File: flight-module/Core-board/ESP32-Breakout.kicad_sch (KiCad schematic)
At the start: 18 parts, among them J10 USB4105-GF-A, J3 Probe_points, SW1 1825910-6, SW2 1825910-6, U10 ESP32-S3-WROOM-1-N16R2, U9 AZ1084-3.3

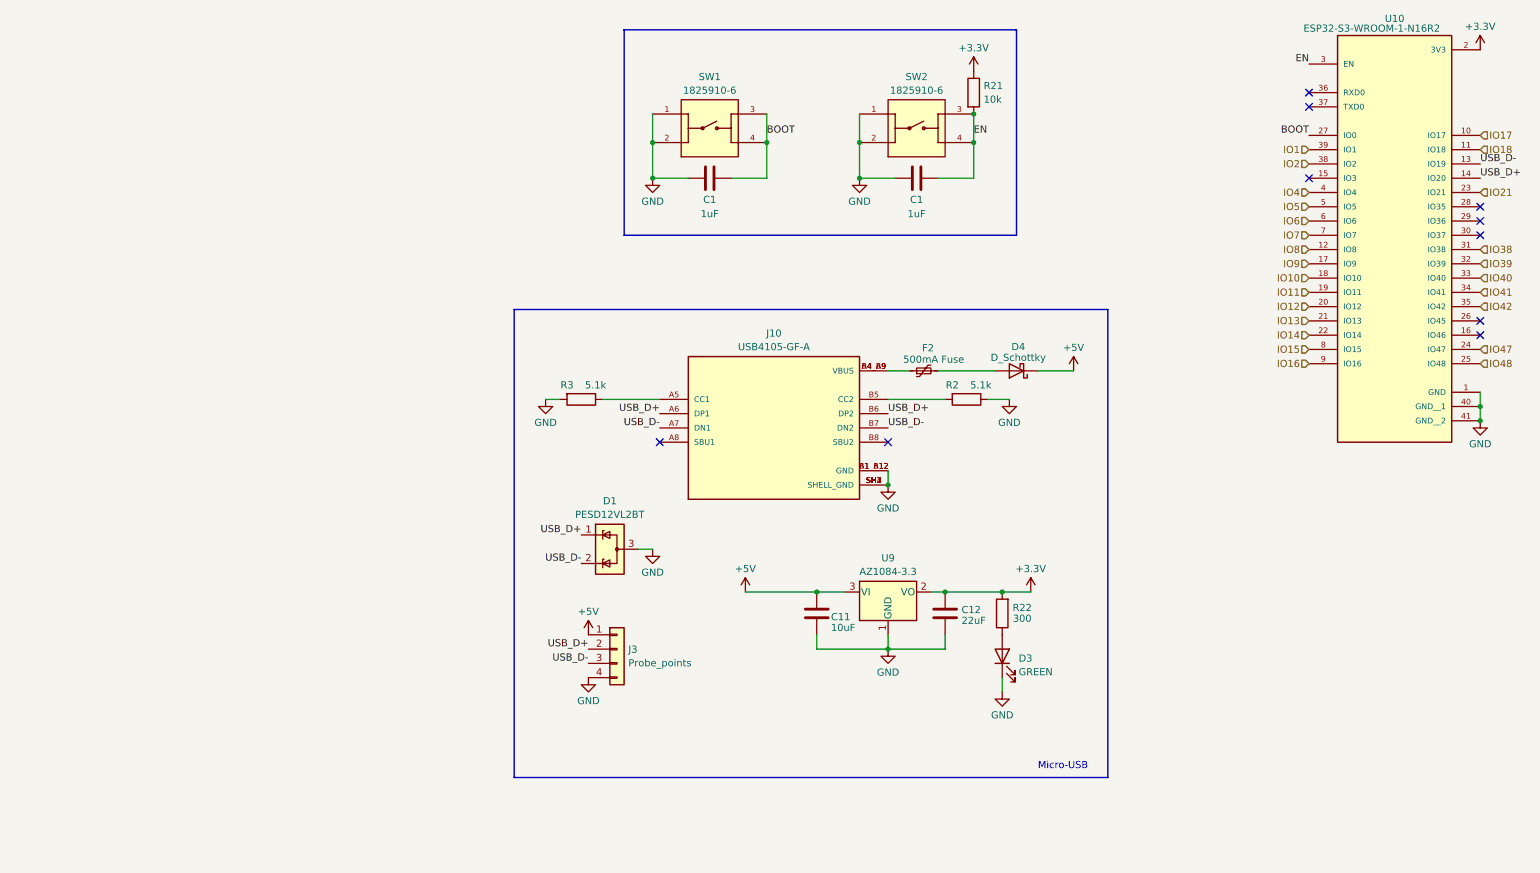
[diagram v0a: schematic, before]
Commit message: in the middle of updating micro usb
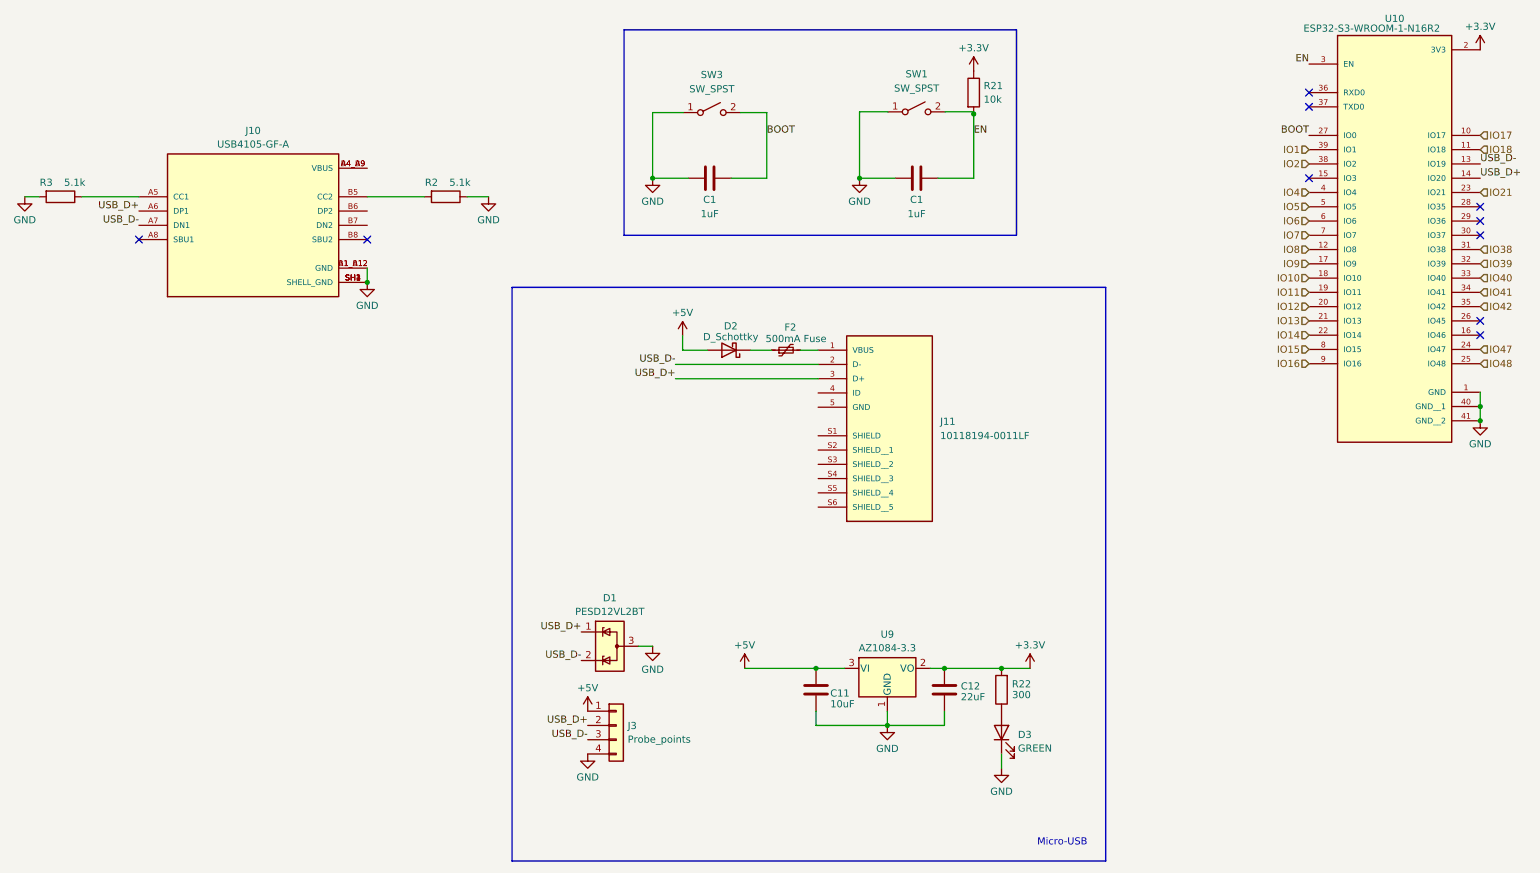
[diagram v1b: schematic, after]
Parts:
- removed D4: D_Schottky, Diode_SMD:D_SOD-128, symbol Device:D_Schottky
- removed SW1, SW2: 1825910-6, 1825910-6:SW_1825910-6-4, symbol 1825910-6:1825910-6
- added D2: D_Schottky, Diode_SMD:D_SOD-128, symbol Device:D_Schottky
- added J11: 10118194-0011LF, 10118194-0011LF:AMPHENOL_10118194-0011LF, symbol MicroUSB:10118194-0011LF
- added SW1, SW3: SW_SPST, Button_Switch_THT:SW_PUSH_6mm, symbol Switch:SW_SPST
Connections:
- net +5V: now also D2.2 (A)
- net BOOT: now also SW3.2 (B)
- net EN: now also SW1.2 (B)
- net GND: now also SW1.1 (A), SW3.1 (A)
- net USB_D+: now also J11.3 (D+); no longer J10.B6 (DP2)
- net USB_D-: now also J11.2 (D-); no longer J10.B7 (DN2)
- net at F2.2: now also J11.1 (VBUS)
- net at J10.A4_B9 (VBUS), J10.B4_A9 (VBUS): no longer F2.1
- new net: D2.1 (K), F2.1
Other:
- moved on the sheet: C11, C12, D1, D3, J10, J3, R2, R22, R3, U9
